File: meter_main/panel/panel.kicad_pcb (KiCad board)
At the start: 2 copper layers, 104 x 102 mm, 100 parts, among them J1 ADC, J2 USB_CDC, J3 HOST_PROG, Q1 S8050, U1 ESP32-S3-WROOM-1, U2 AMS1117/WL9005P3

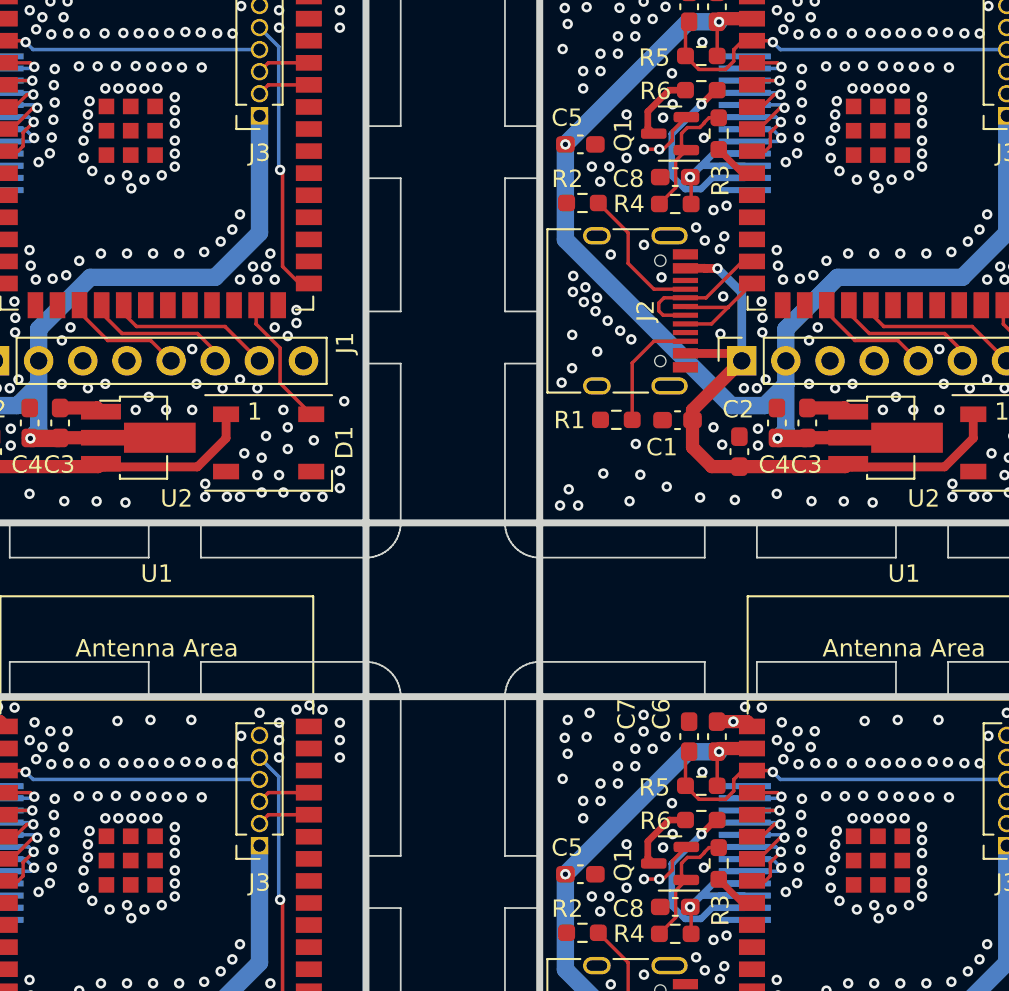
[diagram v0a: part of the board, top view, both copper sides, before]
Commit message: Generate Rev. 1 gerber
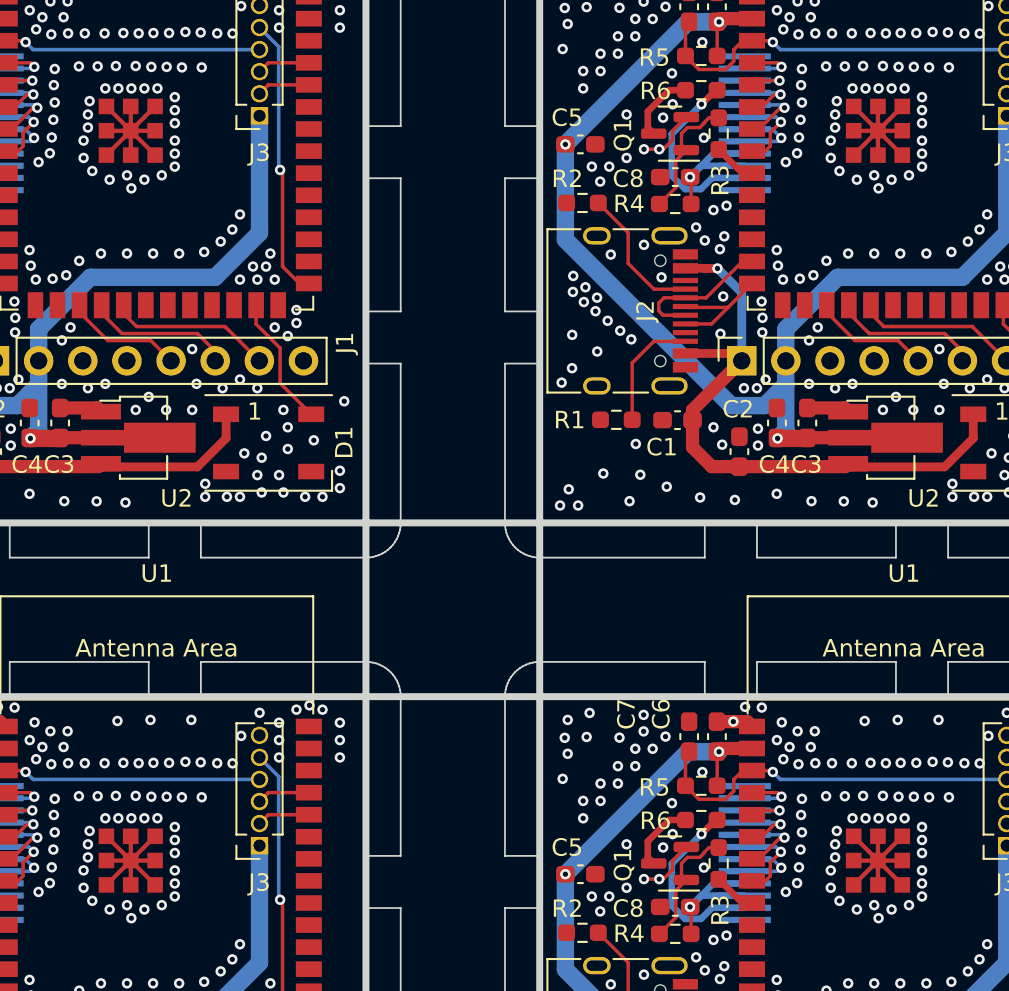
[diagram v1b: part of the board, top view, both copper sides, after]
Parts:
- removed the REF** at (105.5, 24.0) (x2)
- removed the REF** at (105.5, 112.0) (x2)
- removed the REF** at (191.5, 24.0) (x2)
- removed the REF** at (191.5, 112.0) (x2)
- added REF**: Fiducial, Fiducial, F.Cu at (105.5, 24.0)
- added REF**: Fiducial, Fiducial, B.Cu at (105.5, 112.0)
- added REF**: Fiducial, Fiducial, B.Cu at (105.5, 24.0)
- added REF**: Fiducial, Fiducial, B.Cu at (191.5, 112.0)
- added REF**: Fiducial, Fiducial, F.Cu at (191.5, 112.0)
- added REF**: Fiducial, Fiducial, F.Cu at (191.5, 24.0)
- added REF**: Fiducial, Fiducial, F.Cu at (105.5, 112.0)
- added REF**: Fiducial, Fiducial, B.Cu at (191.5, 24.0)
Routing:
- net Board_1-GND: track 12.6 -> 26.1 mm
- net Board_0-GND: track 12.6 -> 26.1 mm
- net Board_2-GND: track 12.6 -> 26.1 mm
- net Board_3-GND: track 12.6 -> 26.1 mm
